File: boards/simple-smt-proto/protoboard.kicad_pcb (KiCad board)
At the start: 2 copper layers, 50 x 50 mm, 1755 parts, among them P1 PAD, P10 PAD, P11 PAD, P12 PAD, P13 PAD, P14 PAD, P15 PAD, P16 PAD, P17 PAD, P18 PAD, P19 PAD, P2 PAD, P20 PAD, P21 PAD, P22 PAD, P23 PAD, P24 PAD, P25 PAD, P26 PAD, P27 PAD, P28 PAD, P29 PAD, P3 PAD, P30 PAD, P31 PAD, P32 PAD, P33 PAD, P34 PAD, P35 PAD, P36 PAD, P37 PAD, P38 PAD, P39 PAD, P4 PAD, P40 PAD, P41 PAD, P42 PAD, P43 PAD, P44 PAD, P45 PAD, P5 PAD, P6 PAD, P7 PAD, P8 PAD, P9 PAD, U1 PROTO_SOIC6, U10 PROTO_SOT23, U100 PAD, U1000 PAD, U1001 PAD, U1002 PAD, U1003 PAD, U1004 PAD, U1005 PAD, U1006 PAD, U1007 PAD, U1008 PAD, U1009 PAD, U101 PAD, U1010 PAD, U1011 PAD, U1012 PAD, U1013 PAD, U1014 PAD, U1015 PAD, U1016 PAD, U1017 PAD, U1018 PAD, U1019 PAD, U102 PAD, U1020 PAD, U1021 PAD, U1022 PAD, U1023 PAD, U1024 PAD, U1025 PAD, U1026 PAD, U1027 PAD, U1028 PAD, U1029 PAD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

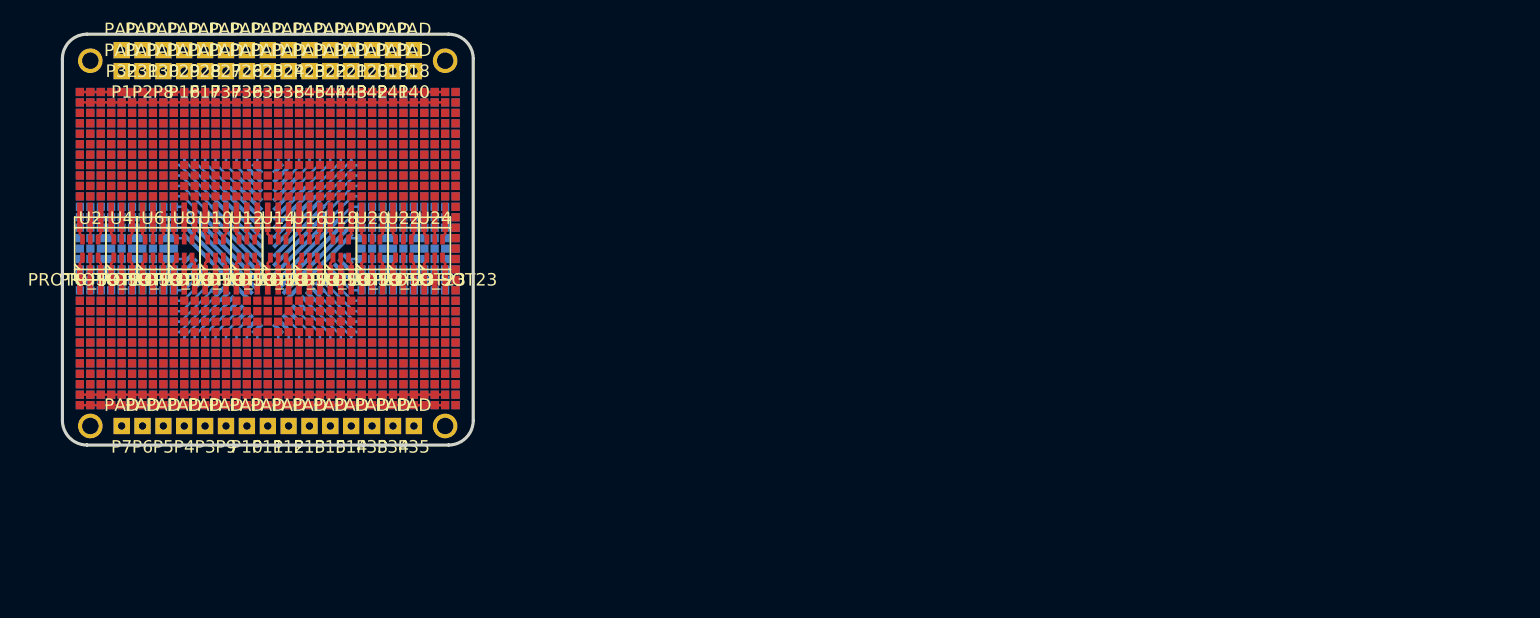
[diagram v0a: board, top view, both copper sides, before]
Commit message: revise smt proto
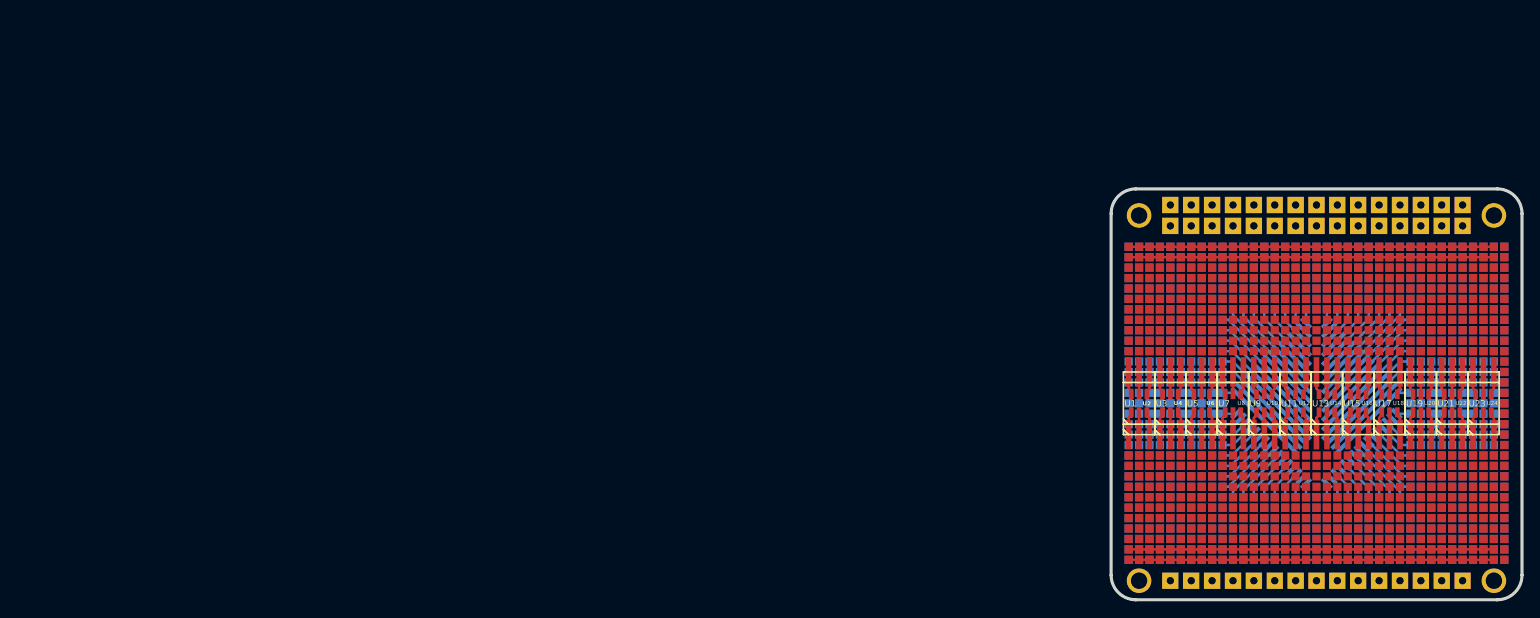
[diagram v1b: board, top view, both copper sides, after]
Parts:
- moved H2 129.0 mm to (199.2, 91.5)
- moved H4 129.0 mm to (199.2, 47.1)
- moved P15 129.0 mm to (185.2, 91.5)
- moved P16 129.0 mm to (167.5, 48.3)
- moved P18 129.0 mm to (195.4, 45.8)
- moved P22 129.0 mm to (185.2, 45.8)
- moved P29 129.0 mm to (167.5, 45.8)
- moved P35 129.0 mm to (195.4, 91.5)
- moved P4 129.0 mm to (167.5, 91.5)
- moved P40 129.0 mm to (195.4, 48.3)
- moved P44 129.0 mm to (185.2, 48.3)
- moved PT25 129.0 mm to (167.5, 58.5)
- moved PT28 129.0 mm to (171.3, 58.5)
- moved PT35 129.0 mm to (181.4, 58.5)
- moved PT38 129.0 mm to (185.2, 58.5)
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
